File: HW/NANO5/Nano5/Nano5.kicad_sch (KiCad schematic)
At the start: 171 parts, among them J1 Screw_Terminal_01x03, J10 Screw_Terminal_01x03, J11 Screw_Terminal_01x03, J12 Screw_Terminal_01x02, J13 Conn_02x04_Counter_Clockwise, J14 Conn_02x04_Counter_Clockwise, J15 Conn_02x03_Counter_Clockwise, J16 Conn_01x02, J17 Conn_01x02, J18 Conn_01x05, J2 Screw_Terminal_01x03, J3 Screw_Terminal_01x03, J4 Screw_Terminal_01x03, J5 Screw_Terminal_01x02, J6 Screw_Terminal_01x02, J7 Screw_Terminal_01x02, J8 Screw_Terminal_01x03, J9 Screw_Terminal_01x03, K1 SANYOU_SRD_Form_C, K2 SANYOU_SRD_Form_C, K3 SANYOU_SRD_Form_C, K4 SANYOU_SRD_Form_C, K5 SANYOU_SRD_Form_C, K6 SANYOU_SRD_Form_C, Q1 MMBT3904, Q10 MMBT3904, Q2 MMBT3904, Q3 MMBT3904, Q4 MMBT3904, Q5 MMBT3904, Q6 MMBT3904, Q7 MMBT3904, Q8 MMBT3904, Q9 MMBT3904, SW1 SW_DIP_x02, U1 ATmega328P-A, U10 ESP-12E, U11 M24C02-RMN, U12 ST485EBDR, U13 DS1307Z+, U14 MP1584, U15 LM358, U16 AP1117-33, U2 LTV-817S, U3 LTV-817S, U4 LTV-817S, U5 LTV-817S, U6 LTV-817S, U7 LTV-817S, U8 LTV-817S, U9 LTV-817S, Y1 Crystal_Small, Y2 Crystal_GND3_Small

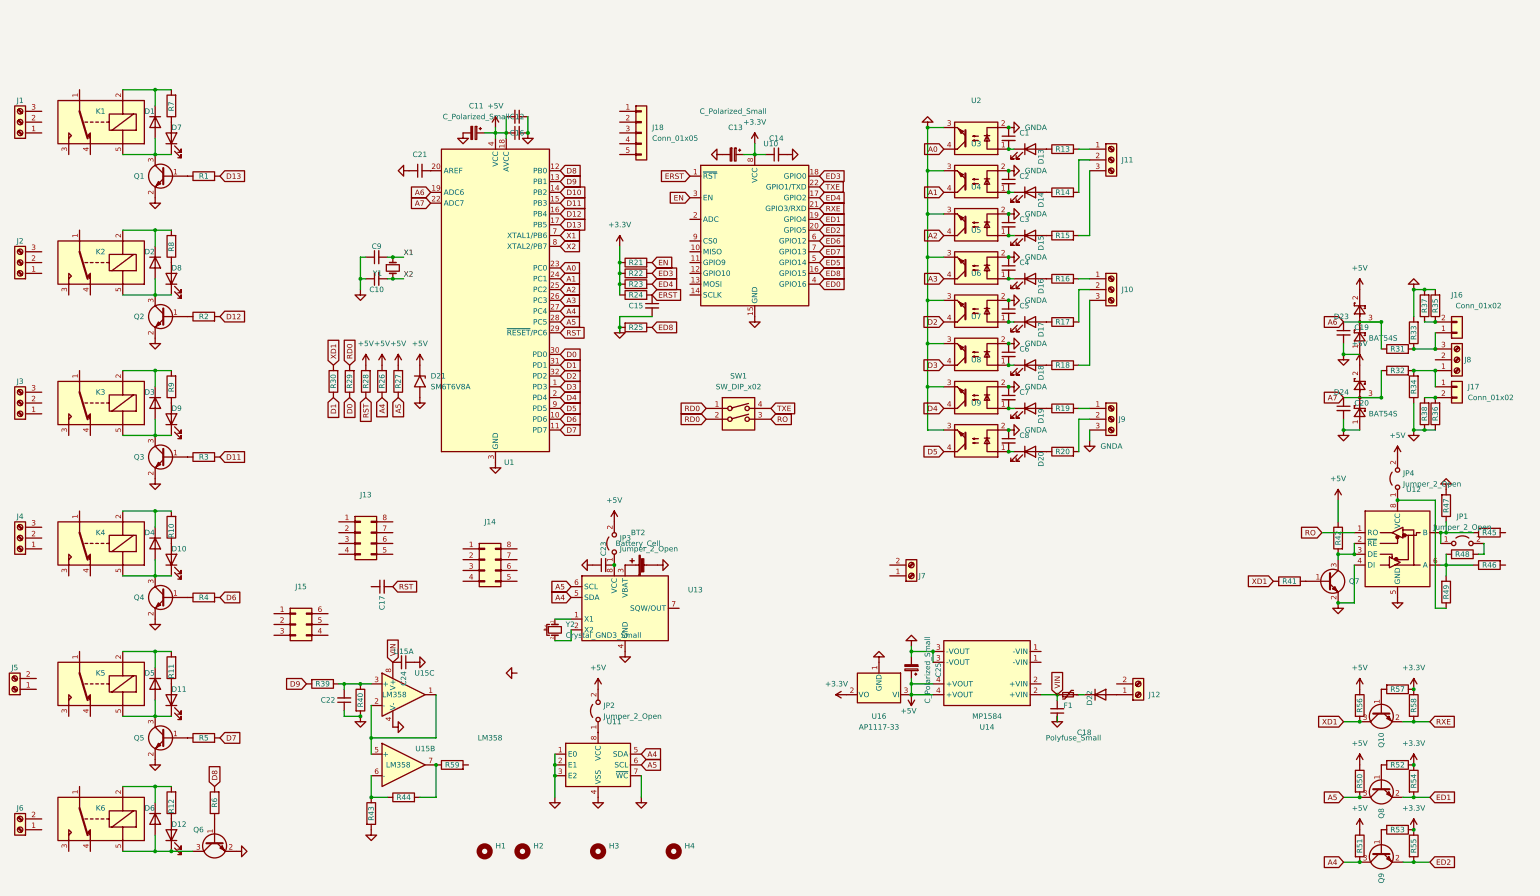
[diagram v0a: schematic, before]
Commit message: update 2104
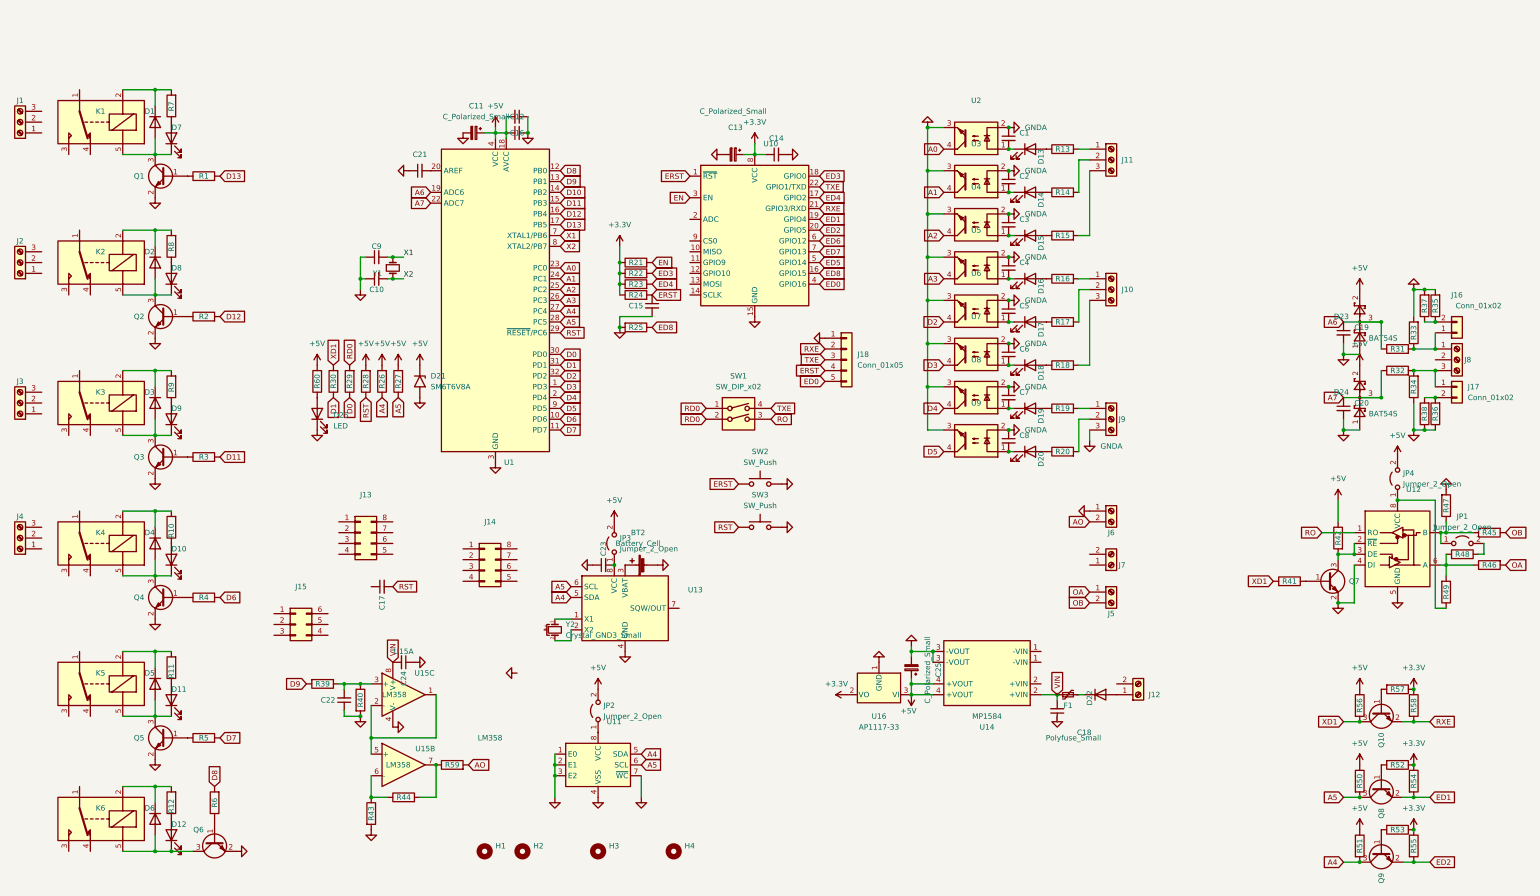
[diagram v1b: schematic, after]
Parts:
- added D25: LED, LED_SMD:LED_0805_2012Metric, symbol Device:LED
- added R60: R, Resistor_SMD:R_0805_2012Metric, symbol Device:R
- added SW2, SW3: SW_Push, Button_Switch_SMD:SW_SPST_B3U-1000P, symbol Switch:SW_Push
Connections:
- net +5V: now also R60.2
- net ED0: now also J18.5 (Pin_5)
- net ERST: now also J18.4 (Pin_4), SW2.1
- net GND: now also J18.1 (Pin_1), J6.1 (Pin_1), D25.1 (K), SW2.2, SW3.2
- net RST: now also SW3.1
- net RXE: now also J18.2 (Pin_2)
- net TXE: now also J18.3 (Pin_3)
- net AO: now reaches J6.2 (Pin_2)
- net AO: now also R59.2
- net OA: now reaches J5.1 (Pin_1)
- net OA: now also R46.2
- net OB: now reaches J5.2 (Pin_2)
- net OB: now also R45.2
- net at J17.1 (Pin_1), R32.2, R34.2: now also J8.3 (Pin_3); no longer J8.1 (Pin_1)
- net at J16.1 (Pin_1), R31.2, R33.1: now also J8.1 (Pin_1); no longer J8.3 (Pin_3)
- new net: D25.2 (A), R60.1
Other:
- moved on the sheet: J18, J5, J6, J7

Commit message: fix update
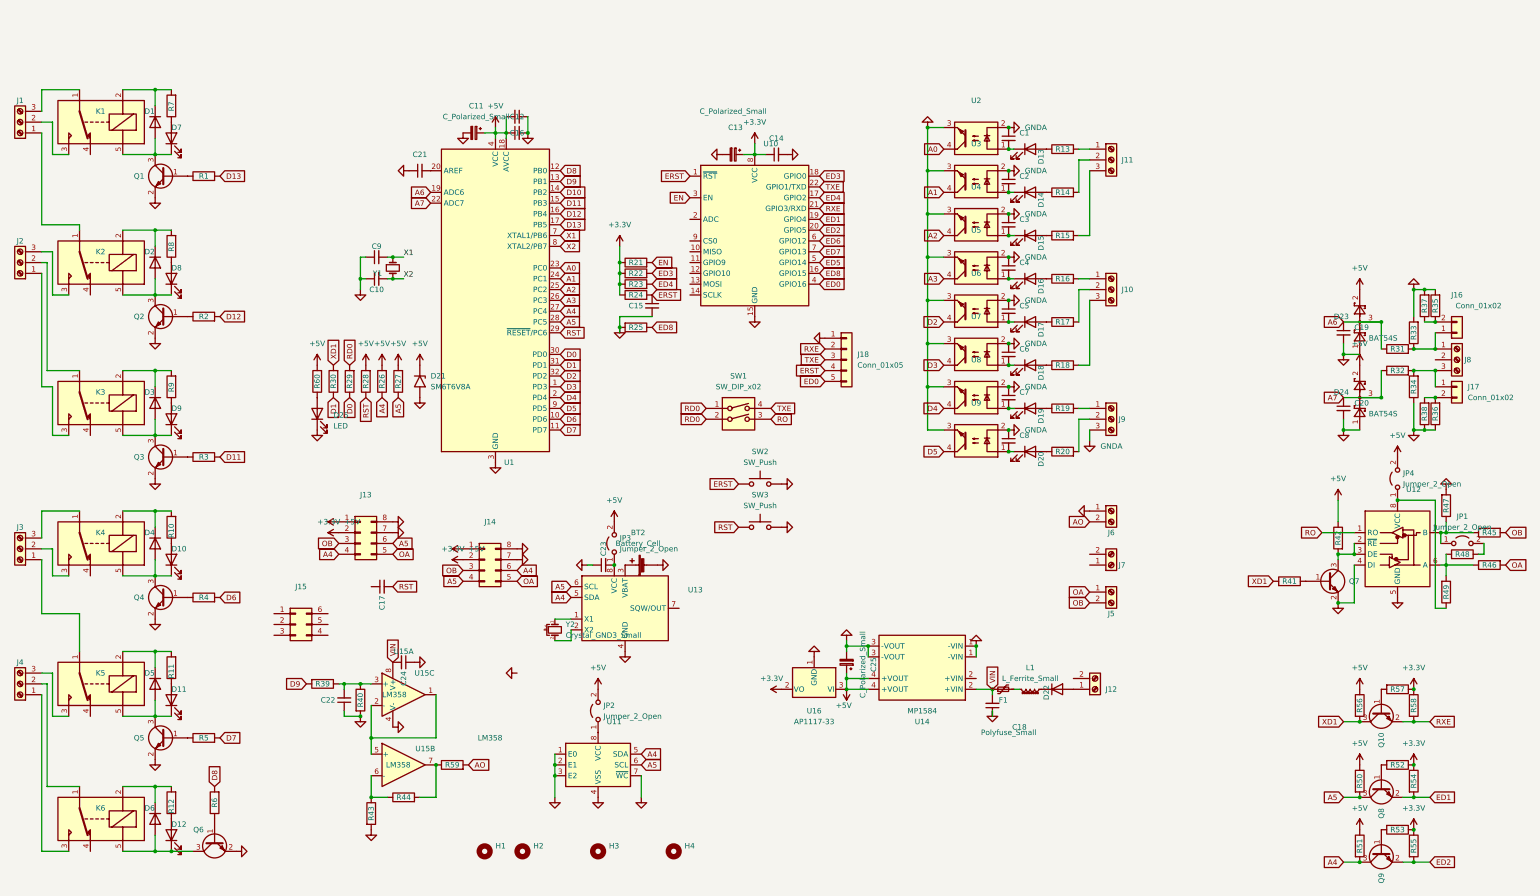
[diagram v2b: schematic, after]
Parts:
- added L1: L_Ferrite_Small, Inductor_SMD:L_1806_4516Metric_Pad1.45x1.90mm_HandSolder, symbol Device:L_Ferrite_Small
- F1: footprint Fuse:Fuse_0805_2012Metric -> Fuse:Fuse_1812_4532Metric
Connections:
- net +3V3: now also J13.2 (Pin_2), J14.2 (Pin_2)
- net +5V: now also J13.1 (Pin_1), J14.1 (Pin_1)
- net A4: now also J13.4 (Pin_4), J14.6 (Pin_6)
- net A5: now also J13.6 (Pin_6), J14.4 (Pin_4)
- net GND: now also J13.7 (Pin_7), J13.8 (Pin_8), J14.7 (Pin_7), J14.8 (Pin_8), U14.1 (-VIN)
- net OA: now also J13.5 (Pin_5), J14.5 (Pin_5)
- net OB: now also J13.3 (Pin_3), J14.3 (Pin_3)
- net at K3.1: now also J2.2 (Pin_2)
- net at K3.3: now also J2.1 (Pin_1)
- net at K5.1: now also J3.1 (Pin_1)
- net at K5.3: now also J4.3 (Pin_3)
- net at K1.1: now also J1.3 (Pin_3)
- net at K1.3: now also J1.2 (Pin_2)
- net at F1.2: now also L1.2; no longer D22.1 (K)
- net at J2.3 (Pin_3): now also K2.3
- net at J3.2 (Pin_2): now also K4.3
- net at J3.3 (Pin_3): now also K4.1
- net at K6.1: now also J4.2 (Pin_2)
- net at K6.3: now also J4.1 (Pin_1)
- net at J1.1 (Pin_1): now also K2.1
- new net: D22.1 (K), L1.1
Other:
- moved on the sheet: C18, C25, D22, F1, J12, J3, J4, U14, U16

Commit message: ISP
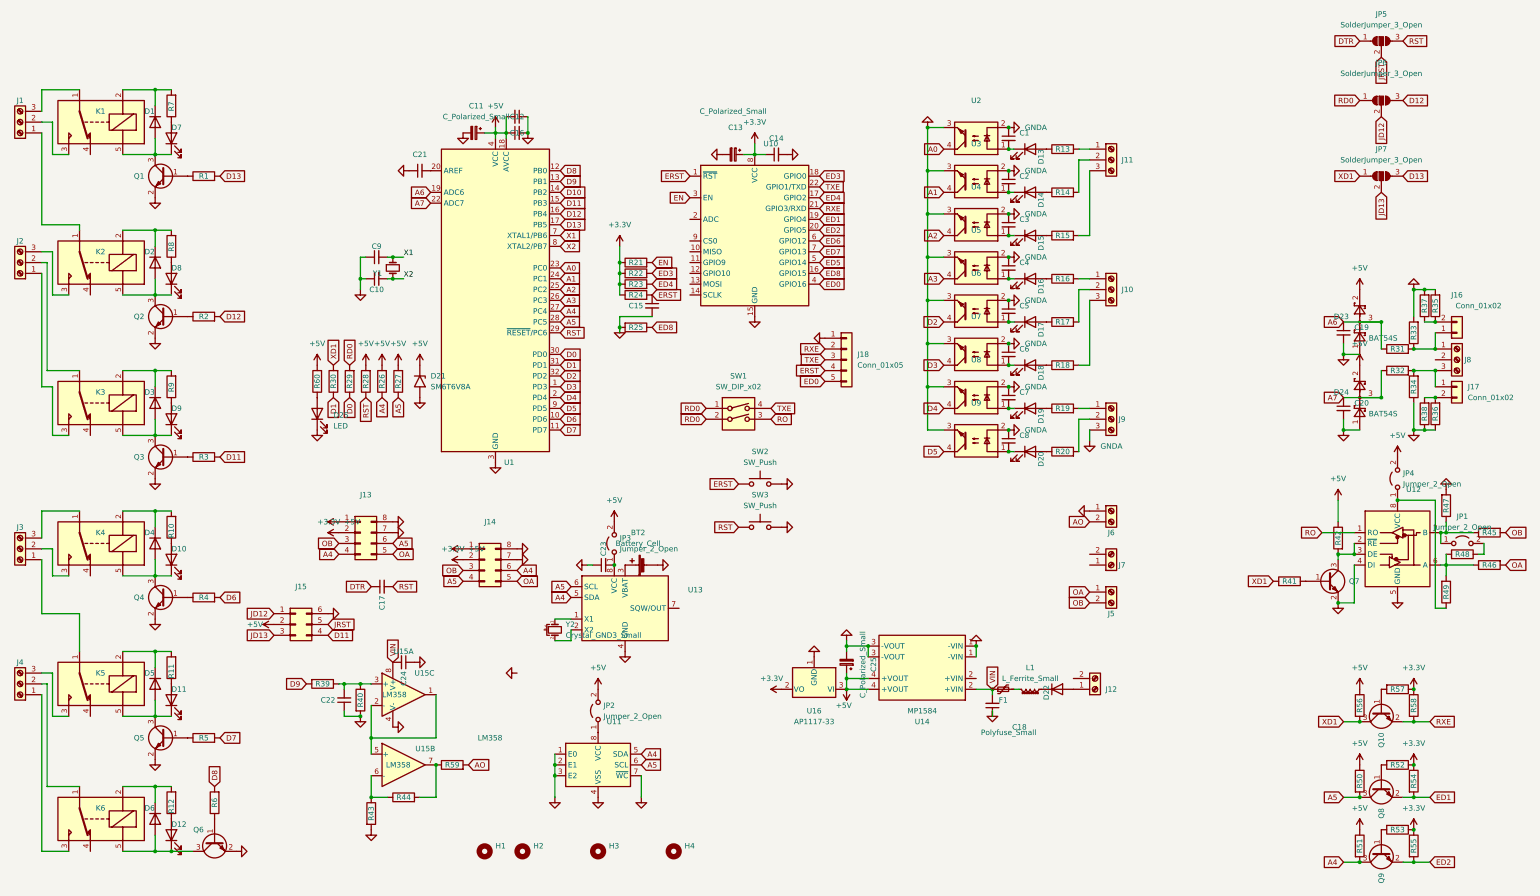
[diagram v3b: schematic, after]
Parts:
- added JP5, JP6, JP7: SolderJumper_3_Open, Jumper:SolderJumper-3_P1.3mm_Open_RoundedPad1.0x1.5mm, symbol Jumper:SolderJumper_3_Open
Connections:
- net +5V: now also J15.2 (Pin_2)
- net D11: now also J15.4 (Pin_4)
- net D12: now also JP6.3 (B)
- net D13: now also JP7.3 (B)
- net GND: now also J15.6 (Pin_6)
- net RD0: now also JP6.1 (A)
- net RST: now also JP5.3 (B)
- net XD1: now also JP7.1 (A)
- net DTR: now reaches C17.1
- net DTR: now also JP5.1 (A)
- net JD12: now reaches J15.1 (Pin_1)
- net JD12: now also JP6.2 (C)
- net JD13: now reaches J15.3 (Pin_3)
- net JD13: now also JP7.2 (C)
- net JRST: now reaches J15.5 (Pin_5)
- net JRST: now also JP5.2 (C)
